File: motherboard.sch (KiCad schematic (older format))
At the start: 0 parts

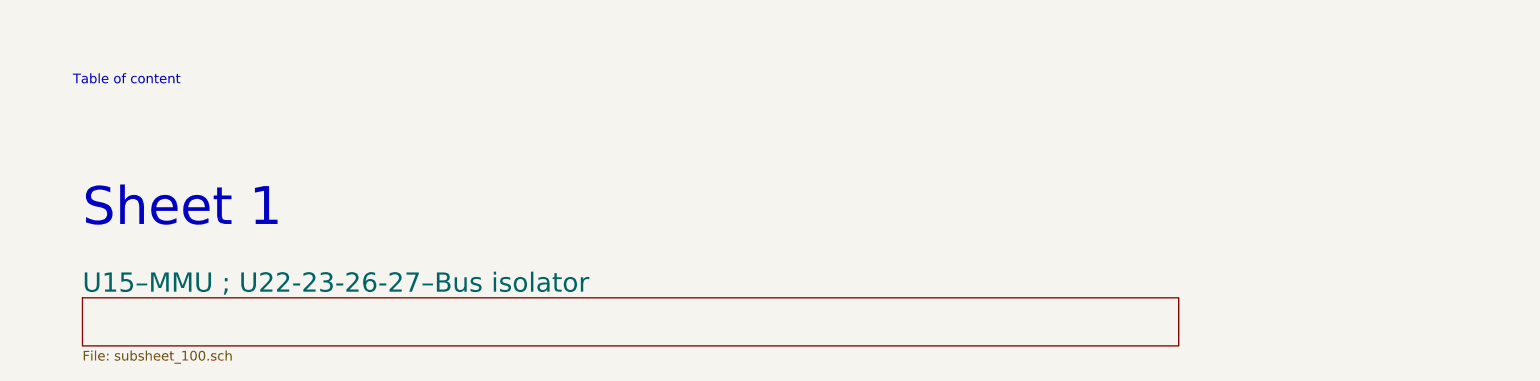
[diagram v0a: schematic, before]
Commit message: reformat main sheet, start fixing directionnality of MMU signals
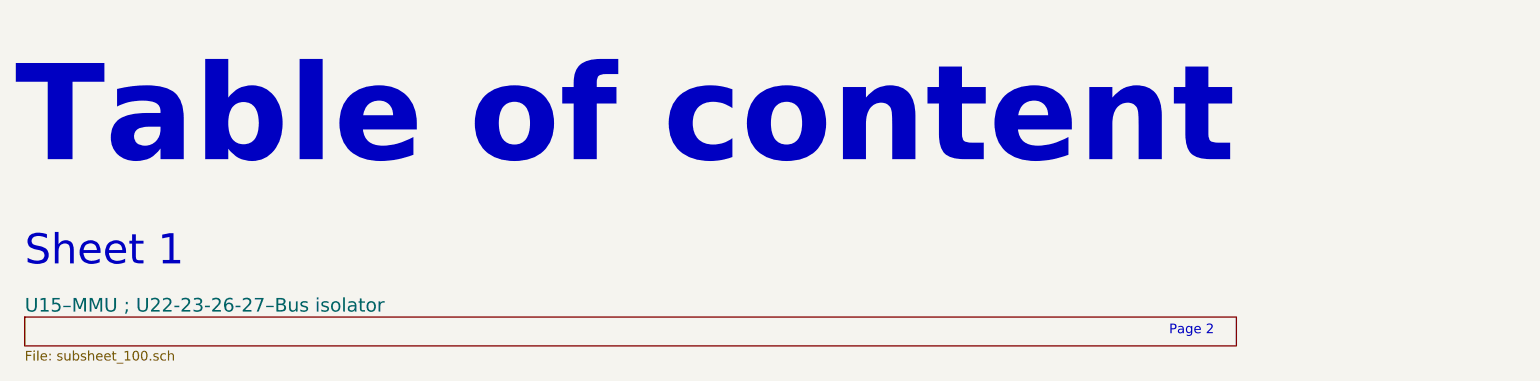
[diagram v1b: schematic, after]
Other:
- note added: "Page 2"
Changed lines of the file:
@@
 Sheet 1 2
 Title "Converted schematics of Atari 260/520 ST"
-Date "2022-07-08"
+Date "2022-07-10"
 Rev "0"
 Comp ""
-Comment1 "Original repository : ---"
-Comment2 "Reference : C070231"
+Comment1 "…sporniket/kicad-conversions--atari-260-520-st-motherboard--c070231"
+Comment2 "Original repository : https://github.com/…"
 Comment3 ""
-Comment4 ""
+Comment4 "Reference : C070231"
 $EndDescr
-Text Notes 1250 1050 0    50   ~ 0
+Text Notes 950  1500 0    500  ~ 100
 Table of content
-Text Notes 1300 1800 0    197  ~ 0
+Text Notes 1000 2000 0    157  ~ 0
 Sheet 1
 $Sheet
-S 1300 2150 5700 250
+S 1000 2250 6300 150
 U 62C842FF
-F0 "U15–MMU ; U22-23-26-27–Bus isolator" 100
+F0 "U15–MMU ; U22-23-26-27–Bus isolator" 71
 F1 "subsheet_100.sch" 50
 $EndSheet
+Text Notes 6950 2350 0    50   ~ 0
+Page 2
 $EndSCHEMATC
